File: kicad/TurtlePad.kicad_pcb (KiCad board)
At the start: 2 copper layers, 108 x 41.3 mm, 23 parts, among them SW1 SW_Push, U1 ProMicro

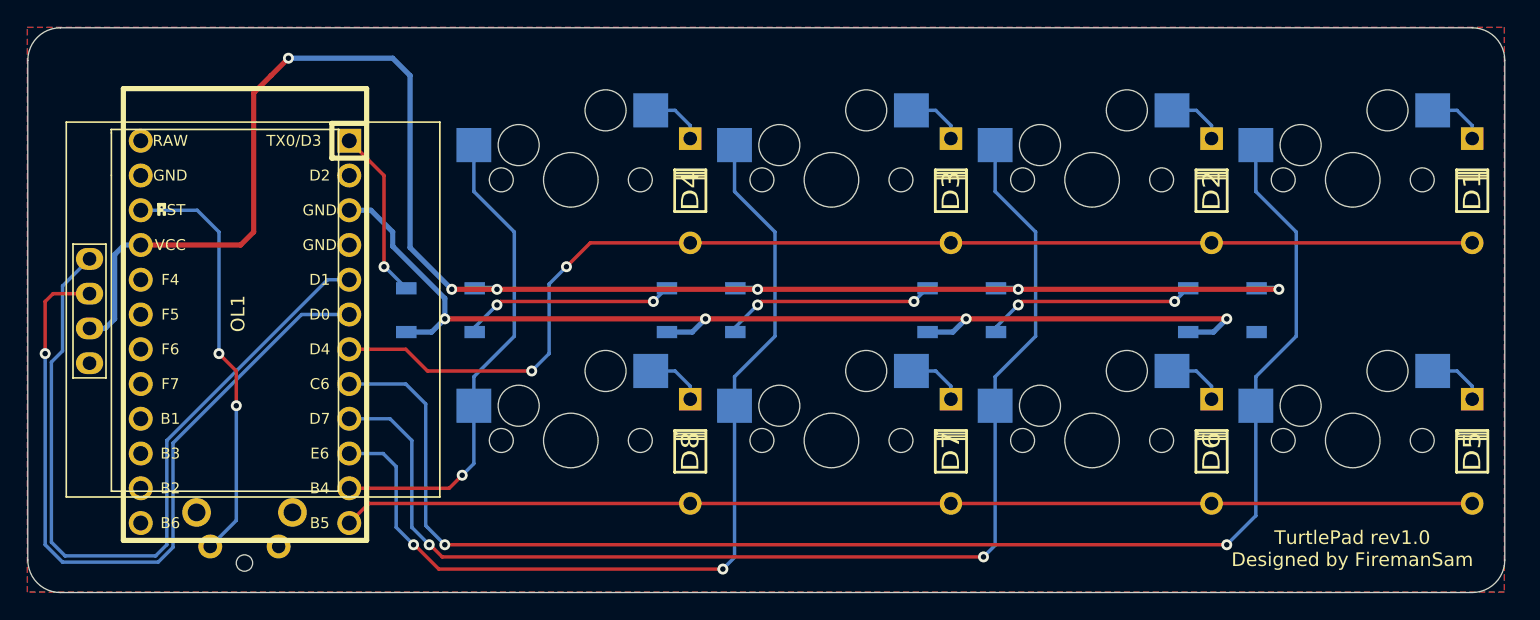
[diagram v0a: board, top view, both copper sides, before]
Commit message: fixed some minor stuff, updated the outline, added solidworks folder for DXFs
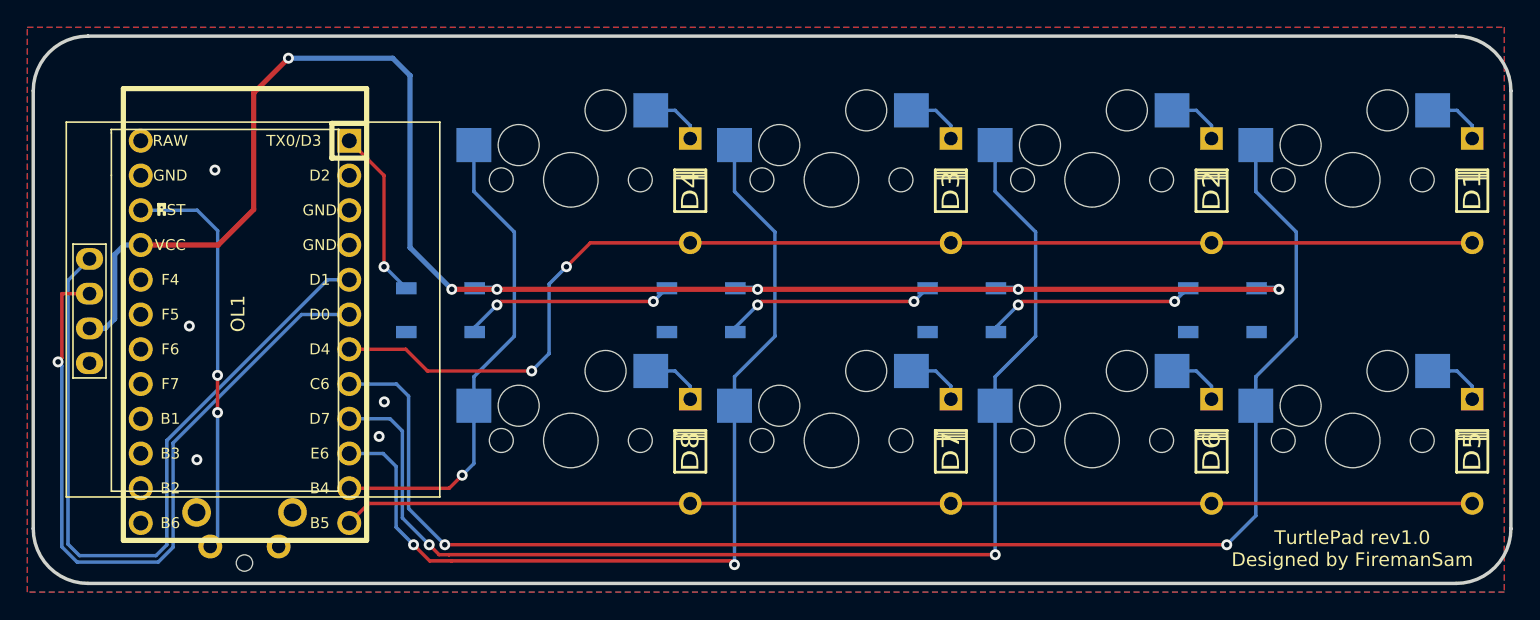
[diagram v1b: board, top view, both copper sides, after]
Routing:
- net GND: track 81.8 -> 0.00 mm, vias 4 -> 5
- net SDA: track 57.6 -> 55.2 mm
- net SCL: track 56.1 -> 54.2 mm
- net reset: track 30.7 -> 29.5 mm
- net VCC: track 124.8 -> 123.9 mm
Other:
- board size 108 x 41.3 mm -> 108 x 40 mm
- net class Default removed
- net class Power removed
